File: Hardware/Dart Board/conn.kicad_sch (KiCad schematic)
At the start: 1 part

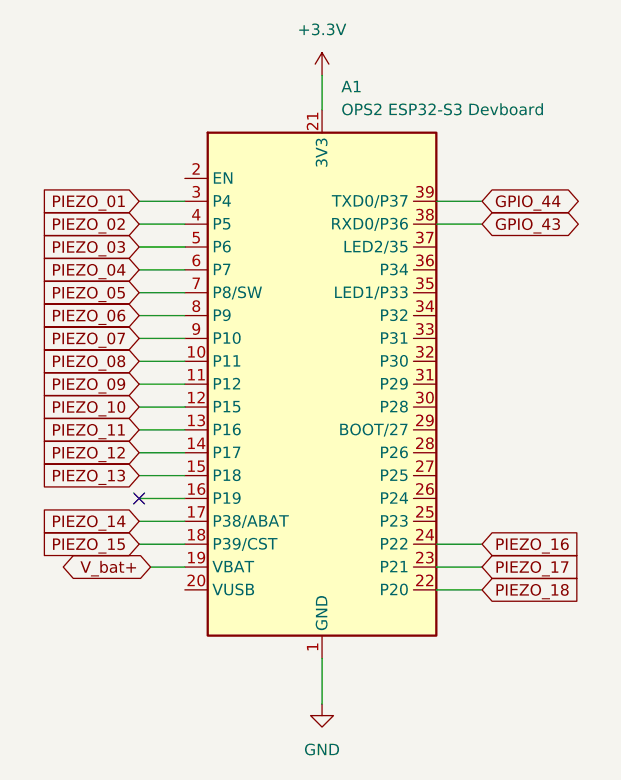
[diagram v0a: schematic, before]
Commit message: Finished PCB Layout
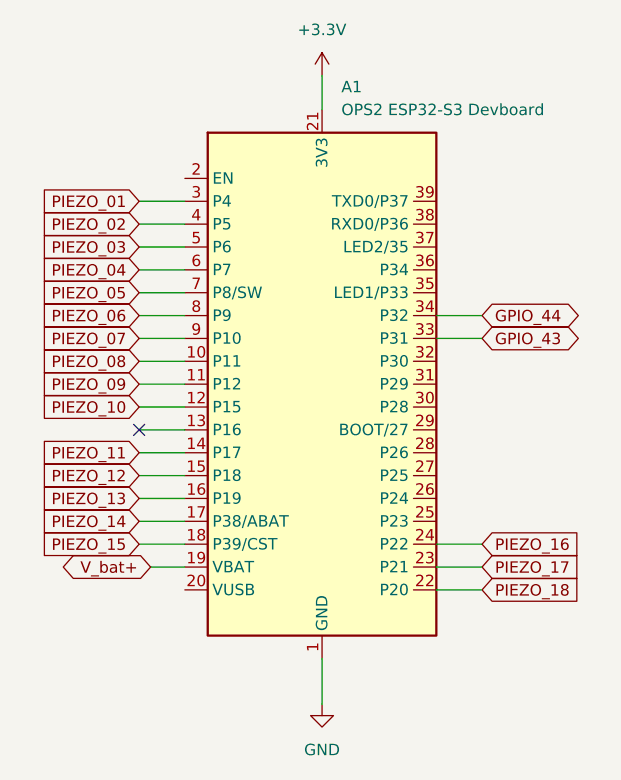
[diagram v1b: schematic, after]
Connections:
- net GPIO_43: now also A1.33 (P31); no longer A1.38 (RXD0/P36)
- net GPIO_44: now also A1.34 (P32); no longer A1.39 (TXD0/P37)
- net PIEZO_11: now also A1.14 (P17); no longer A1.13 (P16)
- net PIEZO_12: now also A1.15 (P18); no longer A1.14 (P17)
- net PIEZO_13: now also A1.16 (P19); no longer A1.15 (P18)
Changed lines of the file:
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@@
 	)
 	(no_connect
-		(at 57.15 102.87)
+		(at 57.15 95.25)
 	)
 	(wire
@@
 	(wire
 		(pts
-			(xy 90.17 69.85) (xy 95.25 69.85)
+			(xy 90.17 82.55) (xy 95.25 82.55)
 		)
 		(stroke
@@
 	(wire
 		(pts
-			(xy 90.17 72.39) (xy 95.25 72.39)
+			(xy 90.17 85.09) (xy 95.25 85.09)
 		)
 		(stroke
@@
 	(global_label "PIEZO_12"
 		(shape input)
-		(at 57.15 97.79 180)
-		(fields_autoplaced yes)
-		(effects
-			(font
-				(size 1.27 1.27)
-			)
-			(justify right)
-		)
-		(property "Intersheetrefs" "${INTERSHEET_REFS}"
-			(at 45.2144 97.79 0)
+		(at 57.15 100.33 180)
+		(fields_autoplaced yes)
+		(effects
+			(font
+				(size 1.27 1.27)
+			)
+			(justify right)
+		)
+		(property "Intersheetrefs" "${INTERSHEET_REFS}"
+			(at 45.2144 100.33 0)
 			(effects
 				(font
@@
 	(global_label "PIEZO_13"
 		(shape input)
-		(at 57.15 100.33 180)
-		(fields_autoplaced yes)
-		(effects
-			(font
-				(size 1.27 1.27)
-			)
-			(justify right)
-		)
-		(property "Intersheetrefs" "${INTERSHEET_REFS}"
-			(at 45.2144 100.33 0)
+		(at 57.15 102.87 180)
+		(fields_autoplaced yes)
+		(effects
+			(font
+				(size 1.27 1.27)
+			)
+			(justify right)
+		)
+		(property "Intersheetrefs" "${INTERSHEET_REFS}"
+			(at 45.2144 102.87 0)
 			(effects
 				(font
@@
 	(global_label "GPIO_43"
 		(shape bidirectional)
-		(at 95.25 72.39 0)
+		(at 95.25 85.09 0)
 		(fields_autoplaced yes)
 		(effects
@@
 		)
 		(property "Intersheetrefs" "${INTERSHEET_REFS}"
-			(at 107.2084 72.39 0)
+			(at 107.2084 85.09 0)
 			(effects
 				(font
@@
 	(global_label "PIEZO_11"
 		(shape input)
-		(at 57.15 95.25 180)
-		(fields_autoplaced yes)
-		(effects
-			(font
-				(size 1.27 1.27)
-			)
-			(justify right)
-		)
-		(property "Intersheetrefs" "${INTERSHEET_REFS}"
-			(at 45.2144 95.25 0)
+		(at 57.15 97.79 180)
+		(fields_autoplaced yes)
+		(effects
+			(font
+				(size 1.27 1.27)
+			)
+			(justify right)
+		)
+		(property "Intersheetrefs" "${INTERSHEET_REFS}"
+			(at 45.2144 97.79 0)
 			(effects
 				(font
@@
 	(global_label "GPIO_44"
 		(shape bidirectional)
-		(at 95.25 69.85 0)
+		(at 95.25 82.55 0)
 		(fields_autoplaced yes)
 		(effects
@@
 		)
 		(property "Intersheetrefs" "${INTERSHEET_REFS}"
-			(at 107.2084 69.85 0)
-			(effects
-				(font
+			(at 107.2084 82.55 0)
+			(effects
+				(font
